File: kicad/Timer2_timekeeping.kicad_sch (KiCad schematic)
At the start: 15 parts, among them J1 Conn_01x02, SW1 SW_Push, SW2 SW_Push, SW3 SW_Push, SW4 SW_Push, U1 ATmega32A-P, Y1 Crystal

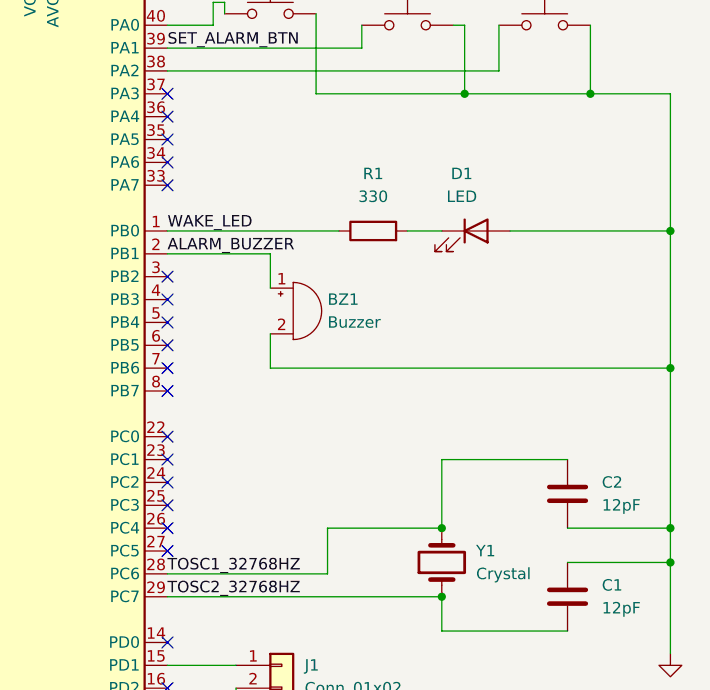
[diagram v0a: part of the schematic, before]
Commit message: small pcb update
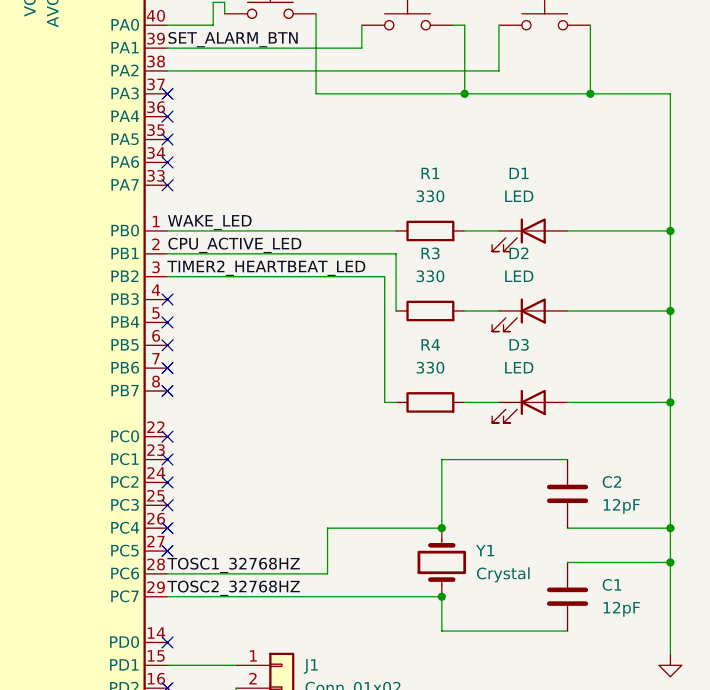
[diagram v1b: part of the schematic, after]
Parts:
- removed BZ1: Buzzer, Buzzer_Beeper:Buzzer_12x9.5RM7.6, symbol Device:Buzzer
- added D2, D3: LED, LED_THT:LED_D5.0mm, symbol Device:LED
- added R3, R4: 330, Resistor_THT:R_Axial_DIN0207_L6.3mm_D2.5mm_P7.62mm_Horizontal, symbol Device:R
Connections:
- net GND: now also D2.2 (A), D3.2 (A)
- net TIMER2_HEARTBEAT_LED: now reaches U1.3 (PB2)
- net TIMER2_HEARTBEAT_LED: now also R4.1
- net ALARM_BUZZER renamed CPU_ACTIVE_LED
- net CPU_ACTIVE_LED: now also R3.1
- new net: D3.1 (K), R4.2
- new net: D2.1 (K), R3.2
- no-connect marks 26 -> 25
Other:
- moved on the sheet: D1, R1
